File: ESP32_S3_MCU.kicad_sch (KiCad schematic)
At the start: 29 parts, among them SW2 SW_Push, SW4 SW_Push, U6 W25Q32JVSS, U8 ESP32-S3, X2 40MHz

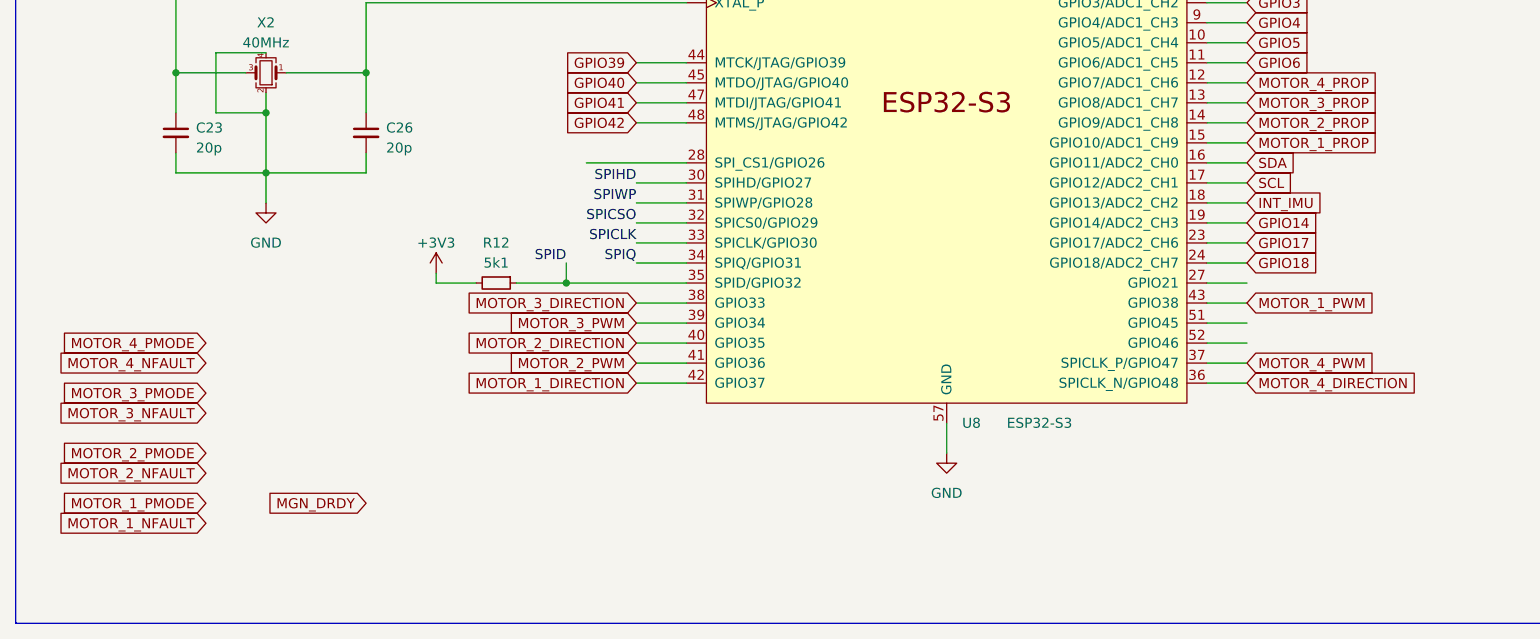
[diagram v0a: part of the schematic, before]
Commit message: checkpoint for backup
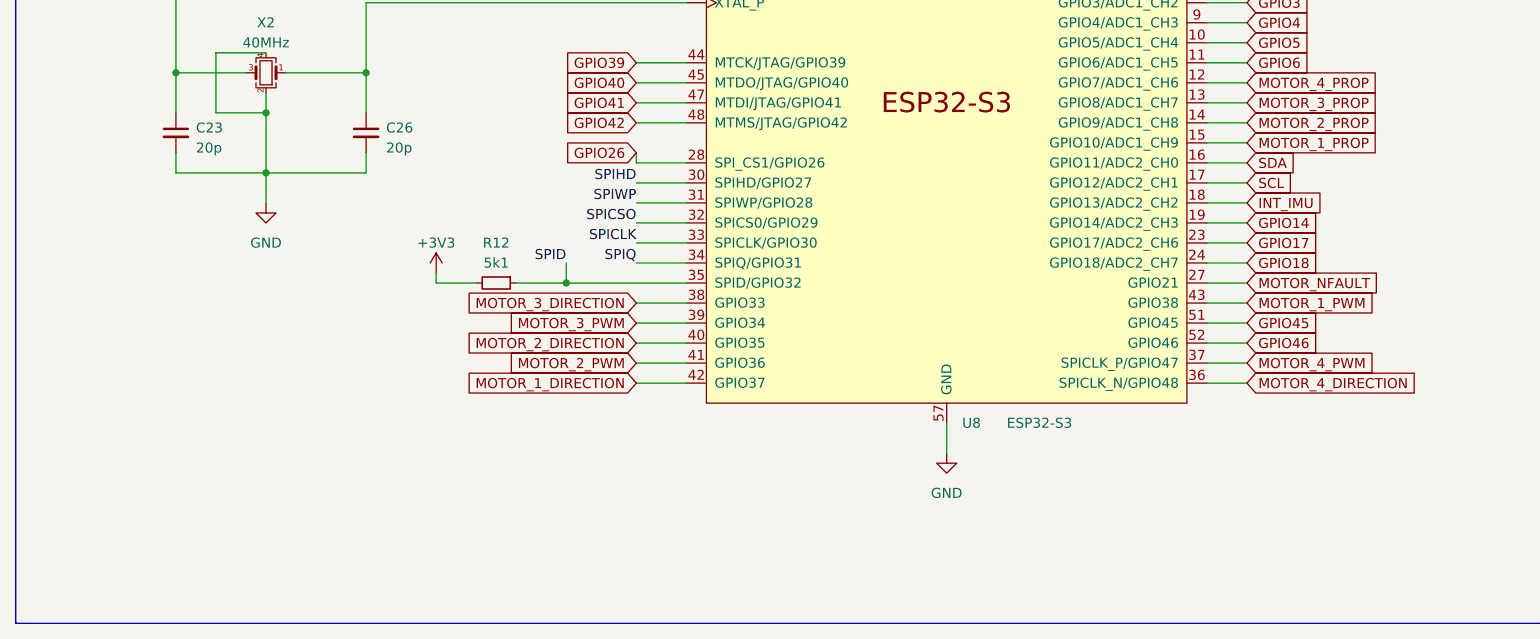
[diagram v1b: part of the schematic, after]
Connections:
- net MOTOR_NFAULT: now reaches U8.27 (GPIO21)
- net GPIO26: now reaches U8.28 (SPI_CS1/GPIO26)
- net GPIO45: now reaches U8.51 (GPIO45)
- net GPIO46: now reaches U8.52 (GPIO46)
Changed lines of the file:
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@@
     (stroke (width 0) (type default))
   )
-  (wire (pts (xy 97.79 158.75) (xy 110.49 158.75))
+  (wire (pts (xy 104.14 158.75) (xy 110.49 158.75))
     (stroke (width 0) (type default))
   )
@@
   )
   (wire (pts (xy 194.31 100.33) (xy 194.31 76.2))
+    (stroke (width 0) (type default))
+  )
+  (wire (pts (xy 104.14 157.48) (xy 104.14 158.75))
     (stroke (width 0) (type default))
   )
@@
     )
   )
-  (global_label "MOTOR_4_NFAULT" (shape input) (at 49.53 184.15 180) (fields_autoplaced)
-    (effects (font (size 1.27 1.27)) (justify right))
-    (property "Intersheetrefs" "${INTERSHEET_REFS}" (at 30.2162 184.15 0)
-      (effects (font (size 1.27 1.27)) (justify right) hide)
-    )
-  )
-  (global_label "MOTOR_1_NFAULT" (shape input) (at 49.53 204.47 180) (fields_autoplaced)
-    (effects (font (size 1.27 1.27)) (justify right))
-    (property "Intersheetrefs" "${INTERSHEET_REFS}" (at 30.2162 204.47 0)
-      (effects (font (size 1.27 1.27)) (justify right) hide)
+  (global_label "MOTOR_NFAULT" (shape input) (at 181.61 173.99 0) (fields_autoplaced)
+    (effects (font (size 1.27 1.27)) (justify left))
+    (property "Intersheetrefs" "${INTERSHEET_REFS}" (at 198.7467 173.99 0)
+      (effects (font (size 1.27 1.27)) (justify left) hide)
     )
   )
@@
     )
   )
-  (global_label "MOTOR_2_NFAULT" (shape input) (at 49.53 198.12 180) (fields_autoplaced)
-    (effects (font (size 1.27 1.27)) (justify right))
-    (property "Intersheetrefs" "${INTERSHEET_REFS}" (at 30.2162 198.12 0)
-      (effects (font (size 1.27 1.27)) (justify right) hide)
-    )
-  )
   (global_label "GPIO3" (shape input) (at 181.61 138.43 0) (fields_autoplaced)
     (effects (font (size 1.27 1.27)) (justify left))
@@
     )
   )
+  (global_label "GPIO26" (shape input) (at 104.14 157.48 180) (fields_autoplaced)
+    (effects (font (size 1.27 1.27)) (justify right))
+    (property "Intersheetrefs" "${INTERSHEET_REFS}" (at 94.2605 157.48 0)
+      (effects (font (size 1.27 1.27)) (justify right) hide)
+    )
+  )
   (global_label "MOTOR_2_DIRECTION" (shape input) (at 104.14 181.61 180) (fields_autoplaced)
     (effects (font (size 1.27 1.27)) (justify right))
@@
     )
   )
-  (global_label "MOTOR_2_PMODE" (shape input) (at 49.53 195.58 180) (fields_autoplaced)
-    (effects (font (size 1.27 1.27)) (justify right))
-    (property "Intersheetrefs" "${INTERSHEET_REFS}" (at 30.5792 195.58 0)
-      (effects (font (size 1.27 1.27)) (justify right) hide)
+  (global_label "GPIO46" (shape input) (at 181.61 181.61 0) (fields_autoplaced)
+    (effects (font (size 1.27 1.27)) (justify left))
+    (property "Intersheetrefs" "${INTERSHEET_REFS}" (at 191.4895 181.61 0)
+      (effects (font (size 1.27 1.27)) (justify left) hide)
     )
   )
@@
     )
   )
-  (global_label "MOTOR_1_PMODE" (shape input) (at 49.53 201.93 180) (fields_autoplaced)
-    (effects (font (size 1.27 1.27)) (justify right))
-    (property "Intersheetrefs" "${INTERSHEET_REFS}" (at 30.5792 201.93 0)
-      (effects (font (size 1.27 1.27)) (justify right) hide)
-    )
-  )
-  (global_label "MOTOR_3_NFAULT" (shape input) (at 49.53 190.5 180) (fields_autoplaced)
-    (effects (font (size 1.27 1.27)) (justify right))
-    (property "Intersheetrefs" "${INTERSHEET_REFS}" (at 30.2162 190.5 0)
-      (effects (font (size 1.27 1.27)) (justify right) hide)
-    )
-  )
   (global_label "MOTOR_4_DIRECTION" (shape input) (at 181.61 186.69 0) (fields_autoplaced)
     (effects (font (size 1.27 1.27)) (justify left))
@@
     )
   )
+  (global_label "GPIO45" (shape input) (at 181.61 179.07 0) (fields_autoplaced)
+    (effects (font (size 1.27 1.27)) (justify left))
+    (property "Intersheetrefs" "${INTERSHEET_REFS}" (at 191.4895 179.07 0)
+      (effects (font (size 1.27 1.27)) (justify left) hide)
+    )
+  )
   (global_label "GPIO1" (shape input) (at 181.61 133.35 0) (fields_autoplaced)
     (effects (font (size 1.27 1.27)) (justify left))
@@
     )
   )
-  (global_label "MOTOR_4_PMODE" (shape input) (at 49.53 181.61 180) (fields_autoplaced)
-    (effects (font (size 1.27 1.27)) (justify right))
-    (property "Intersheetrefs" "${INTERSHEET_REFS}" (at 30.5792 181.61 0)
-      (effects (font (size 1.27 1.27)) (justify right) hide)
-    )
-  )
-  (global_label "MOTOR_3_PMODE" (shape input) (at 49.53 187.96 180) (fields_autoplaced)
-    (effects (font (size 1.27 1.27)) (justify right))
-    (property "Intersheetrefs" "${INTERSHEET_REFS}" (at 30.5792 187.96 0)
-      (effects (font (size 1.27 1.27)) (justify right) hide)
-    )
-  )
   (global_label "GPIO40" (shape input) (at 104.14 148.59 180) (fields_autoplaced)
     (effects (font (size 1.27 1.27)) (justify right))
@@
     )
   )
-  (global_label "MGN_DRDY" (shape input) (at 69.85 201.93 180) (fields_autoplaced)
-    (effects (font (size 1.27 1.27)) (justify right))
-    (property "Intersheetrefs" "${INTERSHEET_REFS}" (at 56.9467 201.93 0)
-      (effects (font (size 1.27 1.27)) (justify right) hide)
-    )
-  )

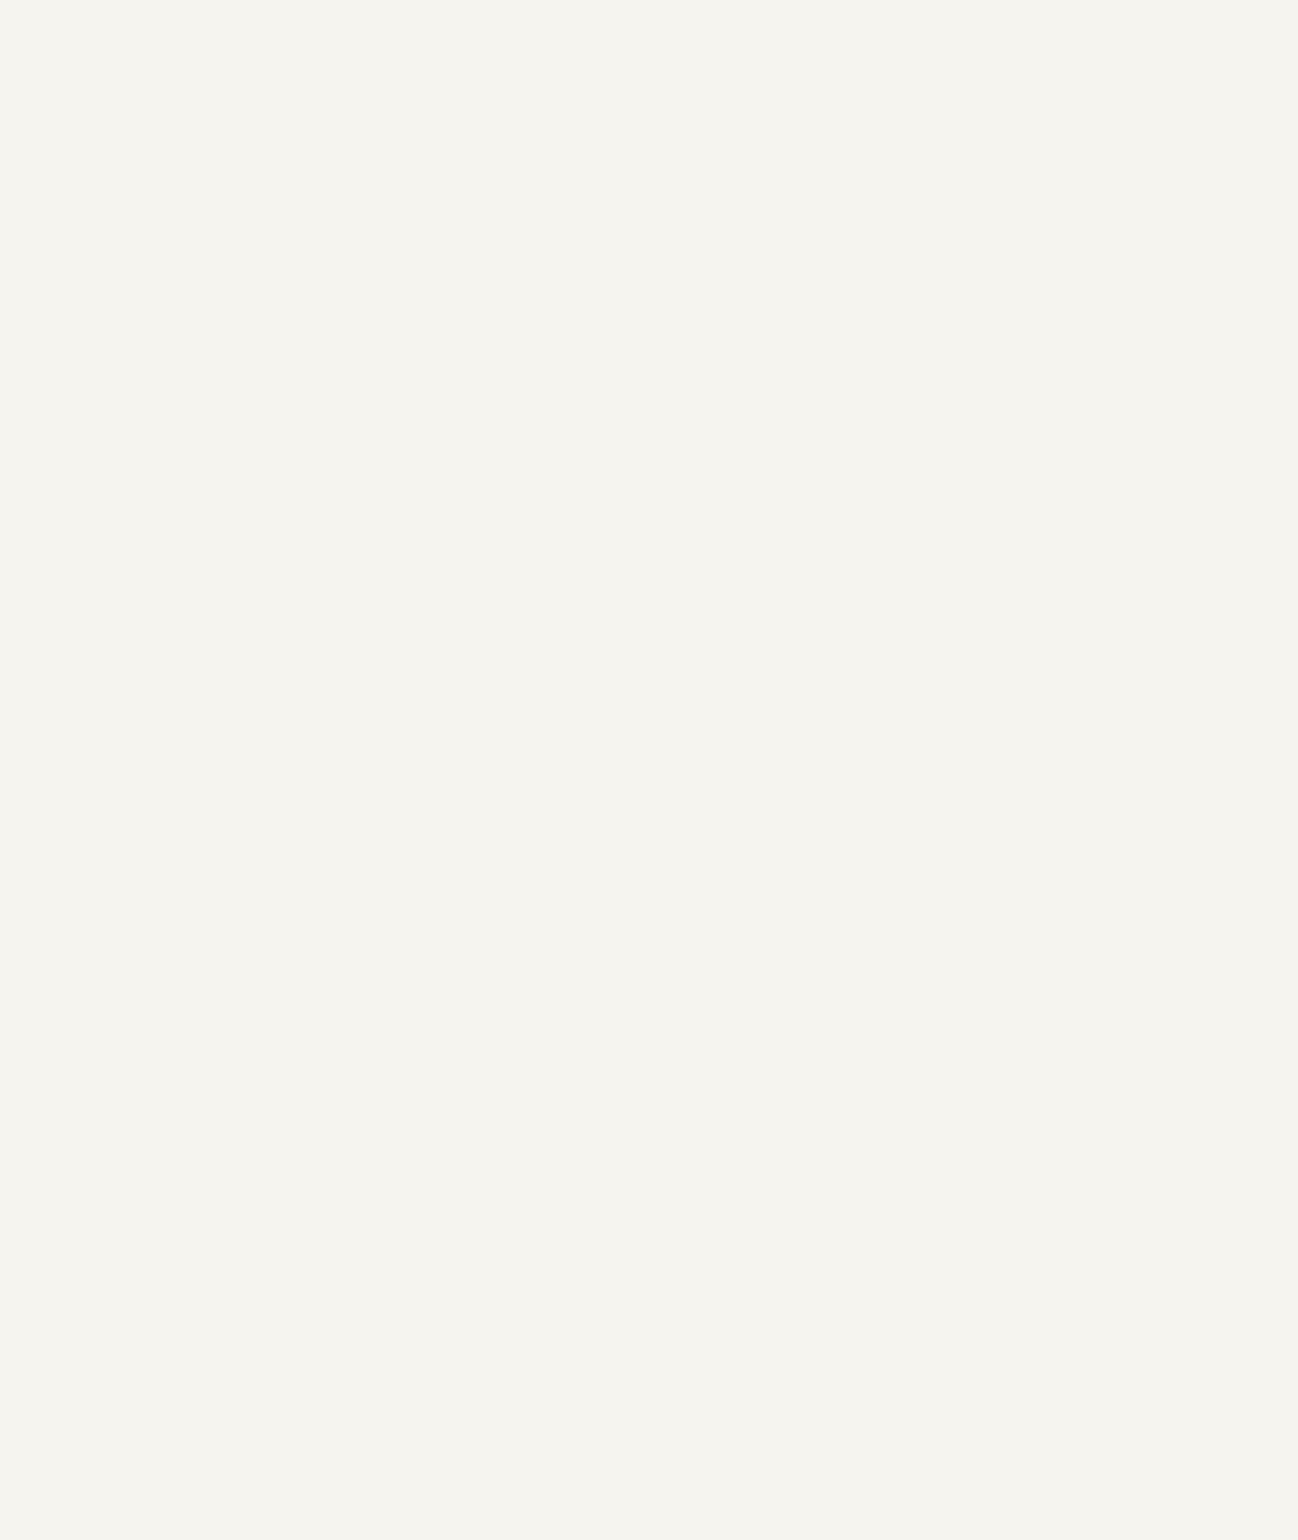
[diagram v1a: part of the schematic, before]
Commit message: Checkpoint before updating MCU
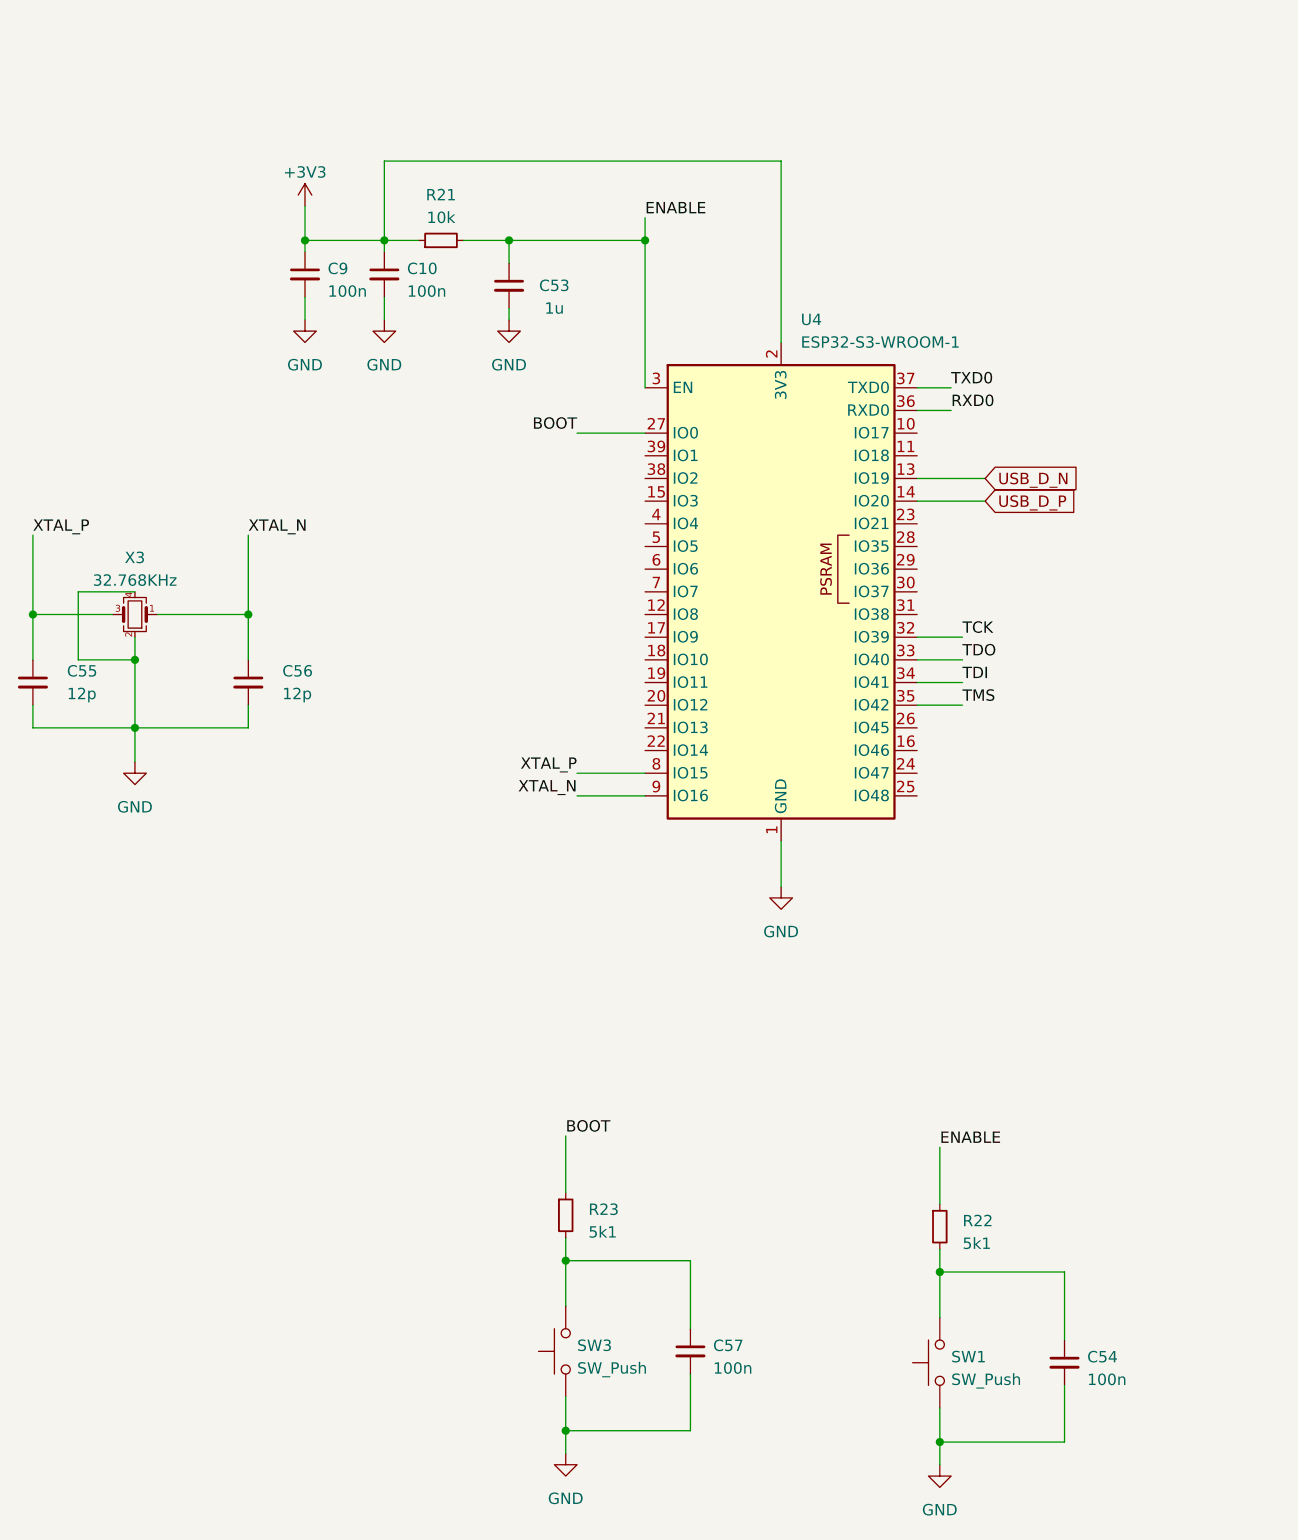
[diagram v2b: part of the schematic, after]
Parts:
- added C10, C54, C57, C9: 100n, Capacitor_SMD:C_0402_1005Metric, symbol Device:C_Small
- added C53: 1u, Capacitor_SMD:C_0402_1005Metric, symbol Device:C_Small
- added C55, C56: 12p, Capacitor_SMD:C_0402_1005Metric, symbol Device:C_Small
- added R21: 10k, symbol Device:R_Small
- added R22, R23: 5k1, Resistor_SMD:R_0603_1608Metric, symbol Device:R_Small
- added SW1, SW3: SW_Push, Button_Switch_SMD:SW_Push_SPST_NO_Alps_SKRK, symbol Switch:SW_Push
- added U4: ESP32-S3-WROOM-1, RF_Module:ESP32-S3-WROOM-1, symbol RF_Module:ESP32-S3-WROOM-1
- added X3: 32.768KHz, Crystal:Crystal_SMD_3225-4Pin_3.2x2.5mm, symbol Device:Crystal_GND24_Small
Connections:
- net +3V3: now also C10.1, C9.1, R21.1, U4.2 (3V3)
- net GND: now also C10.2, C53.2, C54.2, C55.2, C56.2, C57.2, C9.2, SW1.1, SW3.1, U4.1 (GND), U4.40 (GND), U4.41 (GND), X3.2, X3.4
- net USB_D_N: now also U4.13 (IO19)
- net USB_D_P: now also U4.14 (IO20)
- new net: C54.1, R22.2, SW1.2
- new net: C57.1, R23.2, SW3.2
- new net BOOT: R23.1, U4.27 (IO0)
- new net ENABLE: C53.1, R21.2, R22.1, U4.3 (EN)
- new net RXD0: U4.36 (RXD0)
- new net TCK: U4.32 (IO39)
- new net TDI: U4.34 (IO41)
- new net TDO: U4.33 (IO40)
- new net TMS: U4.35 (IO42)
- new net TXD0: U4.37 (TXD0)
- new net XTAL_N: C56.1, U4.9 (IO16), X3.1
- new net XTAL_P: C55.1, U4.8 (IO15), X3.3
